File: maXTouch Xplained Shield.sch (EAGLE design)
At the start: 10 parts, among them IC1 MIC29502BT

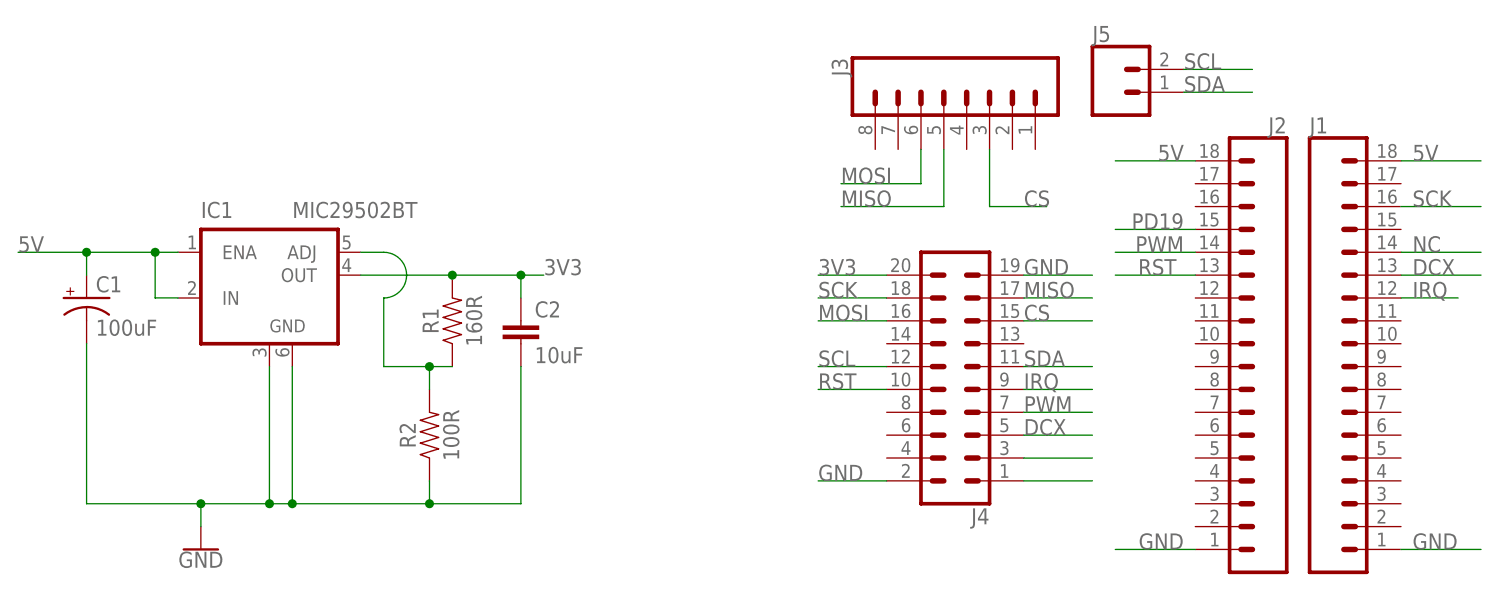
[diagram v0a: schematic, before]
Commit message: THandSMD
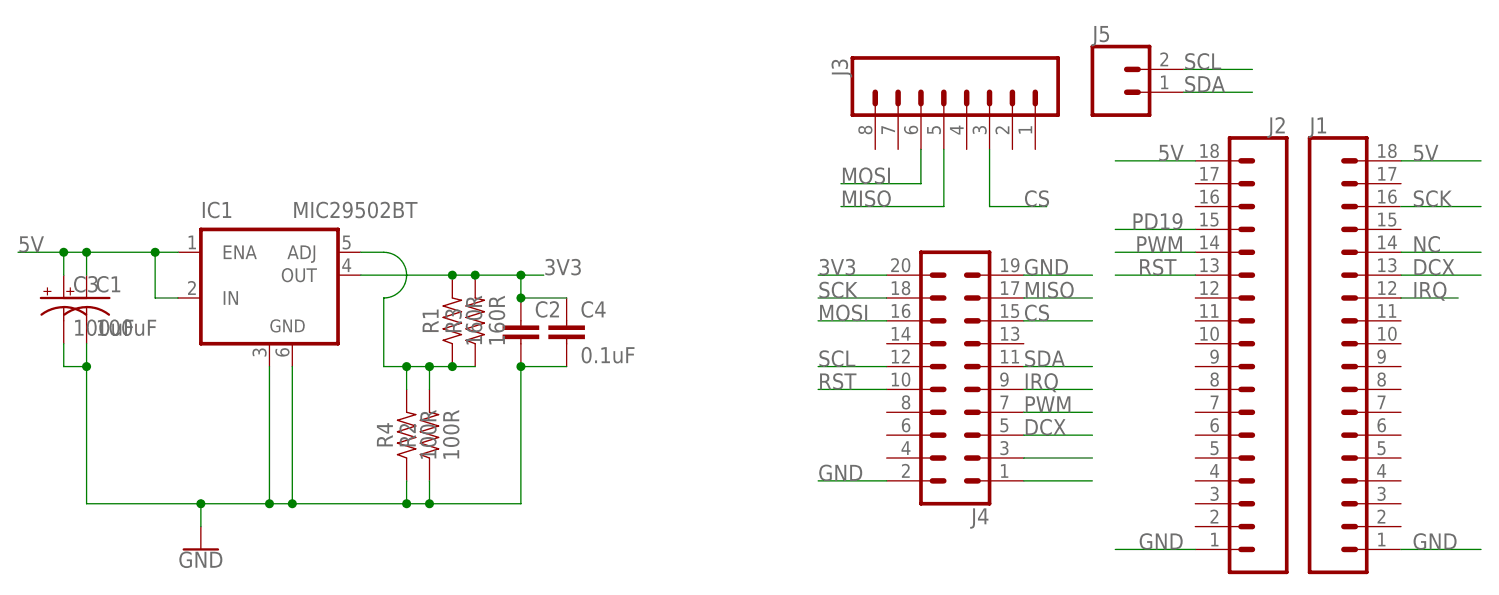
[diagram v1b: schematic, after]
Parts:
- added C3: 100uF, SparkFun-Capacitors:100UF-POLAR-RADIAL-2.5MM-25V-20%
- added C4: 0.1uF, SparkFun-Capacitors:0.1UF-KIT-EZ-50V-20%
- added R3: 160R, SparkFun-Resistors:RESISTORAXIAL-0.3-KIT
- added R4: 100R, SparkFun-Resistors:RESISTORAXIAL-0.3-KIT
- C2: device SparkFun-Capacitors:10UF-0805-10V-10% -> SparkFun-Capacitors:CAP-1206
- R1, R2: device SparkFun-Resistors:RESISTOR0603 -> SparkFun-Resistors:RESISTOR1206
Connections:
- net 3V3: now also C4.1, R3.2
- net 5V: now also C3.+
- net GND: now also C3.-, C4.2, R4.1
- net N$2: now also R3.1, R4.2
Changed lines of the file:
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@@
 <part name="IC1" library="stepper_drivers_etc" deviceset="MIC29502BT" device=""/>
 <part name="C1" library="SparkFun-Capacitors" deviceset="100UF-POLAR" device="-25V-20%(ELEC)" value="100uF"/>
-<part name="R1" library="SparkFun-Resistors" library_urn="urn:adsk.eagle:library:3537822" deviceset="RESISTOR" device="0603" package3d_urn="urn:adsk.eagle:package:3537878/1" value="160R"/>
-<part name="R2" library="SparkFun-Resistors" library_urn="urn:adsk.eagle:library:3537822" deviceset="RESISTOR" device="0603" package3d_urn="urn:adsk.eagle:package:3537878/1" value="100R"/>
-<part name="C2" library="SparkFun-Capacitors" deviceset="10UF" device="-0805-10V-10%" value="10uF"/>
+<part name="R1" library="SparkFun-Resistors" deviceset="RESISTOR" device="1206" value="160R"/>
+<part name="R2" library="SparkFun-Resistors" deviceset="RESISTOR" device="1206" value="100R"/>
+<part name="C2" library="SparkFun-Capacitors" deviceset="CAP" device="-1206" value="10uF"/>
 <part name="GND1" library="SparkFun-PowerSymbols" deviceset="GND" device=""/>
+<part name="R3" library="SparkFun-Resistors" deviceset="RESISTOR" device="AXIAL-0.3-KIT" value="160R"/>
+<part name="R4" library="SparkFun-Resistors" deviceset="RESISTOR" device="AXIAL-0.3-KIT" value="100R"/>
+<part name="C3" library="SparkFun-Capacitors" deviceset="100UF-POLAR" device="-RADIAL-2.5MM-25V-20%" value="100uF"/>
+<part name="C4" library="SparkFun-Capacitors" deviceset="0.1UF" device="-KIT-EZ-50V-20%" value="0.1uF"/>
 </parts>
 <sheets>
@@
 <instance part="C2" gate="G$1" x="-2.54" y="104.14" smashed="yes">
 <attribute name="NAME" x="-1.016" y="107.061" size="1.778" layer="95" font="vector"/>
-<attribute name="VALUE" x="-1.016" y="101.981" size="1.778" layer="96" font="vector"/>
 </instance>
 <instance part="GND1" gate="1" x="-38.1" y="81.28" smashed="yes">
 <attribute name="VALUE" x="-38.1" y="81.026" size="1.778" layer="96" align="top-center"/>
+</instance>
+<instance part="R3" gate="G$1" x="-7.62" y="106.68" smashed="yes" rot="R90">
+<attribute name="NAME" x="-9.144" y="106.68" size="1.778" layer="95" font="vector" rot="R90" align="bottom-center"/>
+<attribute name="VALUE" x="-6.096" y="106.68" size="1.778" layer="96" font="vector" rot="R90" align="top-center"/>
+</instance>
+<instance part="R4" gate="G$1" x="-15.24" y="93.98" smashed="yes" rot="R90">
+<attribute name="NAME" x="-16.764" y="93.98" size="1.778" layer="95" font="vector" rot="R90" align="bottom-center"/>
+<attribute name="VALUE" x="-13.716" y="93.98" size="1.778" layer="96" font="vector" rot="R90" align="top-center"/>
+</instance>
+<instance part="C3" gate="G$1" x="-53.34" y="109.22" smashed="yes">
+<attribute name="NAME" x="-52.324" y="109.855" size="1.778" layer="95" font="vector"/>
+<attribute name="VALUE" x="-52.324" y="105.029" size="1.778" layer="96" font="vector"/>
+</instance>
+<instance part="C4" gate="G$1" x="2.54" y="104.14" smashed="yes">
+<attribute name="NAME" x="4.064" y="107.061" size="1.778" layer="95" font="vector"/>
+<attribute name="VALUE" x="4.064" y="101.981" size="1.778" layer="96" font="vector"/>
 </instance>
 </instances>
@@
 <wire x1="-2.54" y1="101.6" x2="-2.54" y2="86.36" width="0.1524" layer="91"/>
 <wire x1="-2.54" y1="86.36" x2="-12.7" y2="86.36" width="0.1524" layer="91"/>
-<wire x1="-12.7" y1="86.36" x2="-27.94" y2="86.36" width="0.1524" layer="91"/>
+<wire x1="-12.7" y1="86.36" x2="-15.24" y2="86.36" width="0.1524" layer="91"/>
+<wire x1="-15.24" y1="86.36" x2="-27.94" y2="86.36" width="0.1524" layer="91"/>
 <wire x1="-27.94" y1="86.36" x2="-30.48" y2="86.36" width="0.1524" layer="91"/>
 <wire x1="-30.48" y1="86.36" x2="-38.1" y2="86.36" width="0.1524" layer="91"/>
 <wire x1="-38.1" y1="86.36" x2="-50.8" y2="86.36" width="0.1524" layer="91"/>
-<wire x1="-50.8" y1="86.36" x2="-50.8" y2="104.14" width="0.1524" layer="91"/>
+<wire x1="-50.8" y1="86.36" x2="-50.8" y2="101.6" width="0.1524" layer="91"/>
 <pinref part="GND1" gate="1" pin="GND"/>
+<wire x1="-50.8" y1="101.6" x2="-50.8" y2="104.14" width="0.1524" layer="91"/>
 <wire x1="-38.1" y1="83.82" x2="-38.1" y2="86.36" width="0.1524" layer="91"/>
 <junction x="-38.1" y="86.36"/>
@@
 <wire x1="-30.48" y1="101.6" x2="-30.48" y2="86.36" width="0.1524" layer="91"/>
 <junction x="-30.48" y="86.36"/>
+<pinref part="R4" gate="G$1" pin="1"/>
+<wire x1="-15.24" y1="88.9" x2="-15.24" y2="86.36" width="0.1524" layer="91"/>
+<junction x="-15.24" y="86.36"/>
+<pinref part="C3" gate="G$1" pin="-"/>
+<wire x1="-53.34" y1="104.14" x2="-53.34" y2="101.6" width="0.1524" layer="91"/>
+<wire x1="-53.34" y1="101.6" x2="-50.8" y2="101.6" width="0.1524" layer="91"/>
+<junction x="-50.8" y="101.6"/>
+<pinref part="C4" gate="G$1" pin="2"/>
+<wire x1="-2.54" y1="101.6" x2="2.54" y2="101.6" width="0.1524" layer="91"/>
+<junction x="-2.54" y="101.6"/>
 </segment>
 </net>
@@
 </segment>
 <segment>
-<wire x1="-10.16" y1="111.76" x2="-2.54" y2="111.76" width="0.1524" layer="91"/>
+<wire x1="-10.16" y1="111.76" x2="-7.62" y2="111.76" width="0.1524" layer="91"/>
 <pinref part="R1" gate="G$1" pin="2"/>
 <pinref part="C2" gate="G$1" pin="1"/>
+<wire x1="-7.62" y1="111.76" x2="-2.54" y2="111.76" width="0.1524" layer="91"/>
 <wire x1="-2.54" y1="111.76" x2="0" y2="111.76" width="0.1524" layer="91"/>
 <wire x1="-2.54" y1="109.22" x2="-2.54" y2="111.76" width="0.1524" layer="91"/>
@@
 <wire x1="-20.32" y1="111.76" x2="-10.16" y2="111.76" width="0.1524" layer="91"/>
 <junction x="-10.16" y="111.76"/>
+<pinref part="R3" gate="G$1" pin="2"/>
+<junction x="-7.62" y="111.76"/>
+<pinref part="C4" gate="G$1" pin="1"/>
+<wire x1="2.54" y1="109.22" x2="-2.54" y2="109.22" width="0.1524" layer="91"/>
+<junction x="-2.54" y="109.22"/>
 </segment>
 </net>
@@
 <pinref part="IC1" gate="G$1" pin="IN"/>
 <wire x1="-43.18" y1="114.3" x2="-50.8" y2="114.3" width="0.1524" layer="91"/>
-<wire x1="-50.8" y1="114.3" x2="-58.42" y2="114.3" width="0.1524" layer="91"/>
+<wire x1="-50.8" y1="114.3" x2="-53.34" y2="114.3" width="0.1524" layer="91"/>
+<wire x1="-53.34" y1="114.3" x2="-58.42" y2="114.3" width="0.1524" layer="91"/>
 <wire x1="-40.64" y1="109.22" x2="-43.18" y2="109.22" width="0.1524" layer="91"/>
 <wire x1="-43.18" y1="109.22" x2="-43.18" y2="114.3" width="0.1524" layer="91"/>
@@
 <junction x="-50.8" y="114.3"/>
 <label x="-58.42" y="114.3" size="1.778" layer="95"/>
+<pinref part="C3" gate="G$1" pin="+"/>
+<wire x1="-53.34" y1="111.76" x2="-53.34" y2="114.3" width="0.1524" layer="91"/>
+<junction x="-53.34" y="114.3"/>
 </segment>
 </net>
@@
 <wire x1="-12.7" y1="99.06" x2="-12.7" y2="101.6" width="0.1524" layer="91"/>
 <wire x1="-12.7" y1="101.6" x2="-10.16" y2="101.6" width="0.1524" layer="91"/>
-<wire x1="-12.7" y1="101.6" x2="-17.78" y2="101.6" width="0.1524" layer="91"/>
+<wire x1="-12.7" y1="101.6" x2="-15.24" y2="101.6" width="0.1524" layer="91"/>
 <junction x="-12.7" y="101.6"/>
 <pinref part="IC1" gate="G$1" pin="ADJ"/>
+<wire x1="-15.24" y1="101.6" x2="-17.78" y2="101.6" width="0.1524" layer="91"/>
 <wire x1="-20.32" y1="114.3" x2="-17.78" y2="114.3" width="0.1524" layer="91"/>
 <wire x1="-17.78" y1="109.22" x2="-17.78" y2="101.6" width="0.1524" layer="91"/>
 <wire x1="-17.78" y1="114.3" x2="-15.24" y2="111.76" width="0.1524" layer="91" curve="-90"/>
 <wire x1="-17.78" y1="109.22" x2="-15.24" y2="111.76" width="0.1524" layer="91" curve="90"/>
-</segment>
-</net>
+<pinref part="R4" gate="G$1" pin="2"/>
+<wire x1="-15.24" y1="99.06" x2="-15.24" y2="101.6" width="0.1524" layer="91"/>
+<junction x="-15.24" y="101.6"/>
+<pinref part="R3" gate="G$1" pin="1"/>
+<wire x1="-10.16" y1="101.6" x2="-7.62" y2="101.6" width="0.1524" layer="91"/>
+<junction x="-10.16" y="101.6"/>
+</segment>
+</net>
